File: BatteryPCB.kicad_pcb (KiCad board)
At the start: 2 copper layers, 142 x 129.8 mm, 6 parts, among them J1 Pack1+, J2 Sense_Pack1, J3 Pack1-, J4 Sense_Pack2, J5 Pack2+, J6 Pack2-

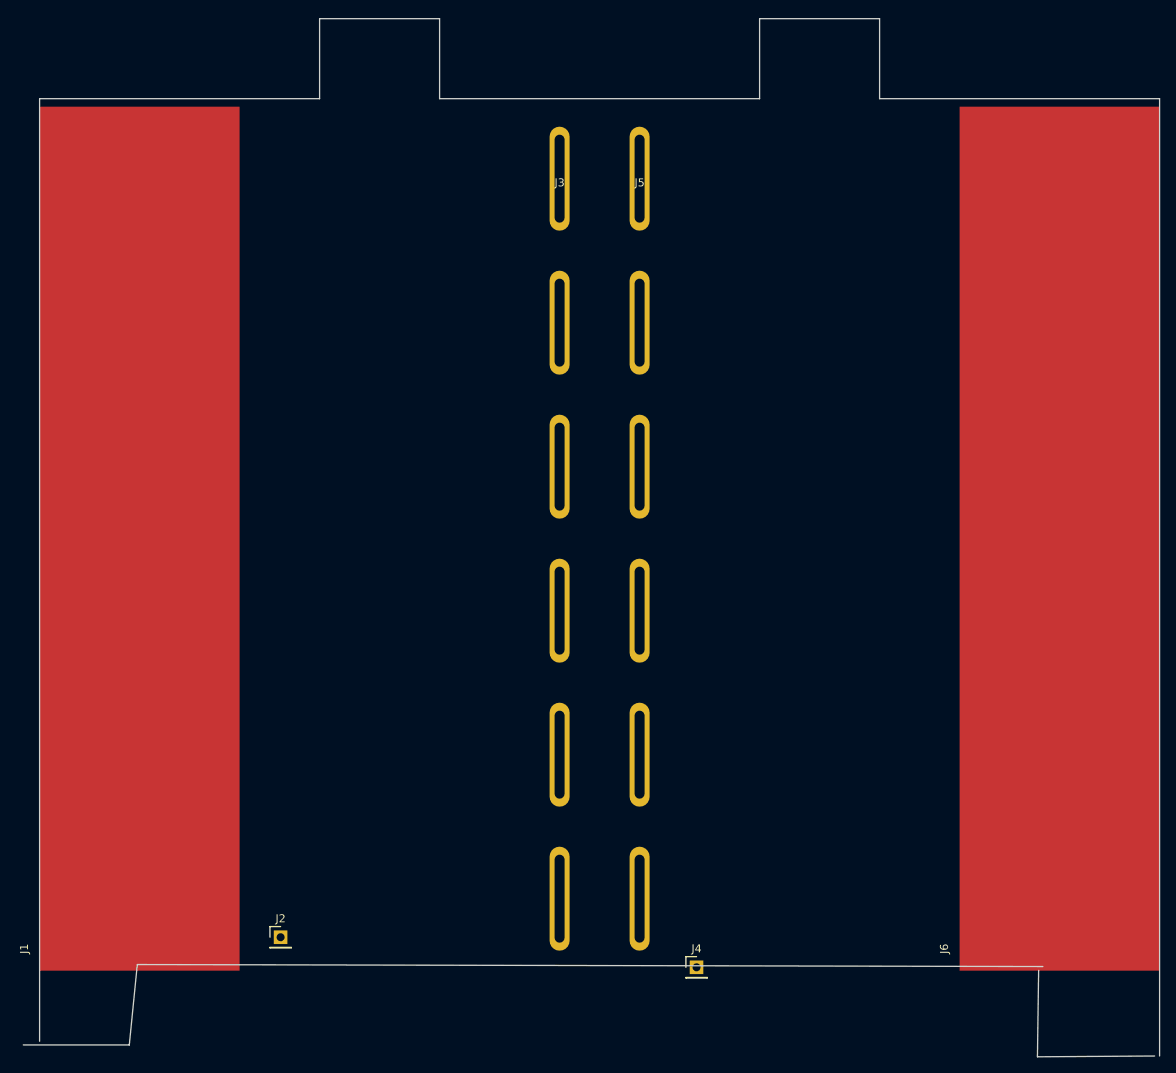
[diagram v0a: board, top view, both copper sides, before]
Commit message: PCB is pretty much done, still need to tweak outline and silkscreen
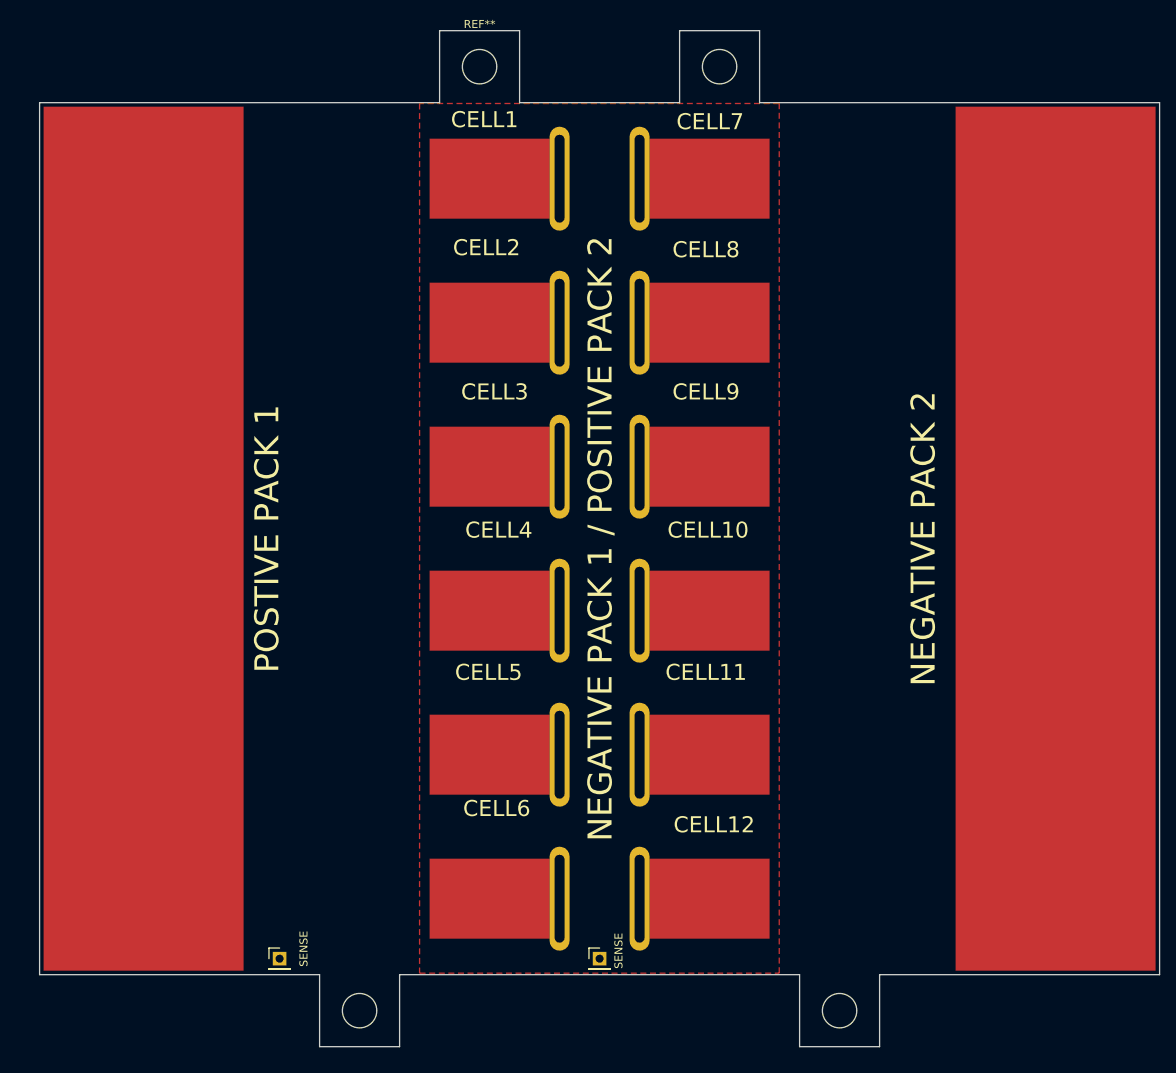
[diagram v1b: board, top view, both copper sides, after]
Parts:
- added REF**: MountingHole_4.3mm_M4, Mounting_Holes:MountingHole_4.3mm_M4, F.Cu at (100.0, 104.0)
- added REF**: MountingHole_4.3mm_M4, Mounting_Holes:MountingHole_4.3mm_M4, F.Cu at (40.0, 104.0)
- added REF**: MountingHole_4.3mm_M4, Mounting_Holes:MountingHole_4.3mm_M4, F.Cu at (55.0, -14.0)
- added REF**: MountingHole_4.3mm_M4, Mounting_Holes:MountingHole_4.3mm_M4, F.Cu at (85.0, -14.0)
- moved J3 90.0 mm to (65.0, 90.0), turned to 180 degrees
- moved J4 12.2 mm to (70.0, 97.5)
- moved J2 2.68 mm to (30.0, 97.5)
- moved J1 0.50 mm to (13.0, 0.00)
- moved J6 0.50 mm to (127.0, 0.00)
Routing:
- added copper zone on F.Cu, net Net-(J3-Pad1)
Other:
- board size 142 x 129.8 mm -> 140 x 127 mm
- board text added: "CELL1"
- board text added: "CELL10"
- board text added: "CELL11"
- board text added: "CELL12"
- board text added: "CELL2"
- board text added: "CELL3"
- board text added: "CELL4"
- board text added: "CELL5"
- board text added: "CELL6"
- board text added: "CELL7"
- board text added: "CELL8"
- board text added: "CELL9"
- board text added: "NEGATIVE PACK 1 / POSITIVE PACK 2"
- board text added: "NEGATIVE PACK 2"
- board text added: "POSTIVE PACK 1"
- board text added: "SENSE"
